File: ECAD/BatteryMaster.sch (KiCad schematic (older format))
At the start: 33 parts

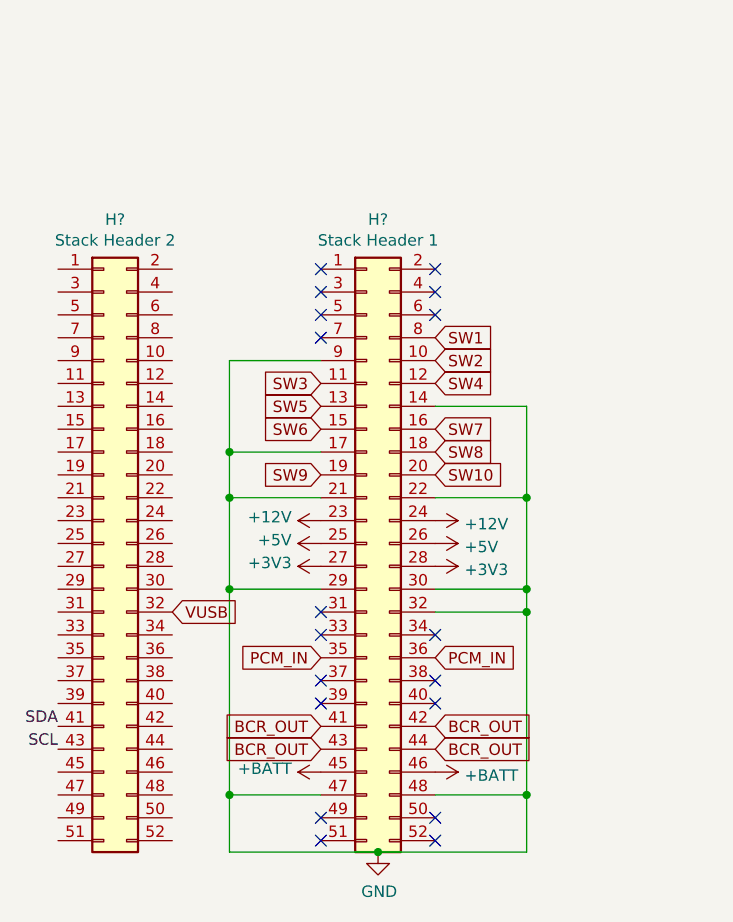
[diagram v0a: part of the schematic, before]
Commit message: rearrange the stack headers to make some damn sense *looks at clydespace*
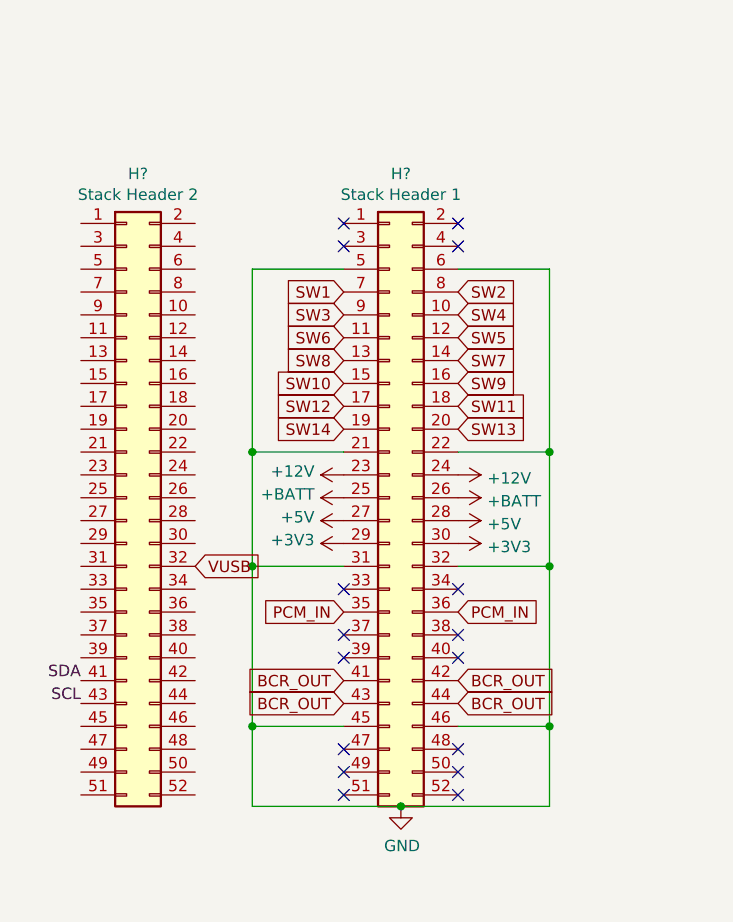
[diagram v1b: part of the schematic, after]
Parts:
- removed H?: Stack Header 2, symbol Connector_Generic:Conn_02x26_Odd_Even
- removed H?: Stack Header 1, symbol Connector_Generic:Conn_02x26_Odd_Even
- added H?: Stack Header 2, symbol Connector_Generic:Conn_02x26_Odd_Even
- added H?: Stack Header 1, symbol Connector_Generic:Conn_02x26_Odd_Even
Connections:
- net +12V: now also H?.23 (Pin_23), H?.24 (Pin_24)
- net +3V3: now also H?.29 (Pin_29), H?.30 (Pin_30)
- net +5V: now also H?.27 (Pin_27), H?.28 (Pin_28)
- net +BATT: now also H?.25 (Pin_25), H?.26 (Pin_26)
- net BCR_OUT: now also H?.41 (Pin_41), H?.42 (Pin_42), H?.43 (Pin_43), H?.44 (Pin_44)
- net GND: now also H?.21 (Pin_21), H?.22 (Pin_22), H?.31 (Pin_31), H?.32 (Pin_32), H?.45 (Pin_45), H?.46 (Pin_46), H?.5 (Pin_5), H?.6 (Pin_6)
- net PCM_IN: now also H?.35 (Pin_35), H?.36 (Pin_36)
- net SCL: now also H?.43 (Pin_43)
- net SDA: now also H?.41 (Pin_41)
- net SW1: now also H?.7 (Pin_7)
- net SW10: now also H?.15 (Pin_15)
- net SW2: now also H?.8 (Pin_8)
- net SW3: now also H?.9 (Pin_9)
- net SW4: now also H?.10 (Pin_10)
- net SW5: now also H?.12 (Pin_12)
- net SW6: now also H?.11 (Pin_11)
- net SW7: now also H?.14 (Pin_14)
- net SW8: now also H?.13 (Pin_13)
- net SW9: now also H?.16 (Pin_16)
- net VUSB: now also H?.32 (Pin_32)
- new net SW11: H?.18 (Pin_18)
- new net SW12: H?.17 (Pin_17)
- new net SW13: H?.20 (Pin_20)
- new net SW14: H?.19 (Pin_19)
- no-connect marks 18 -> 16

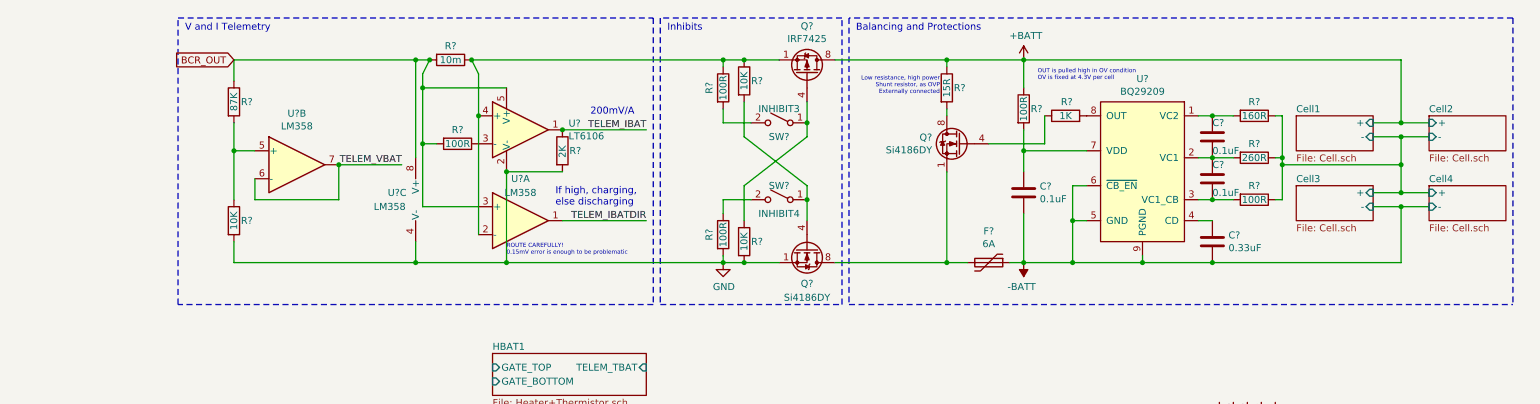
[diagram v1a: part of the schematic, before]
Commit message: spec out new cell protection IC and mosfets, figured out current limit calculation
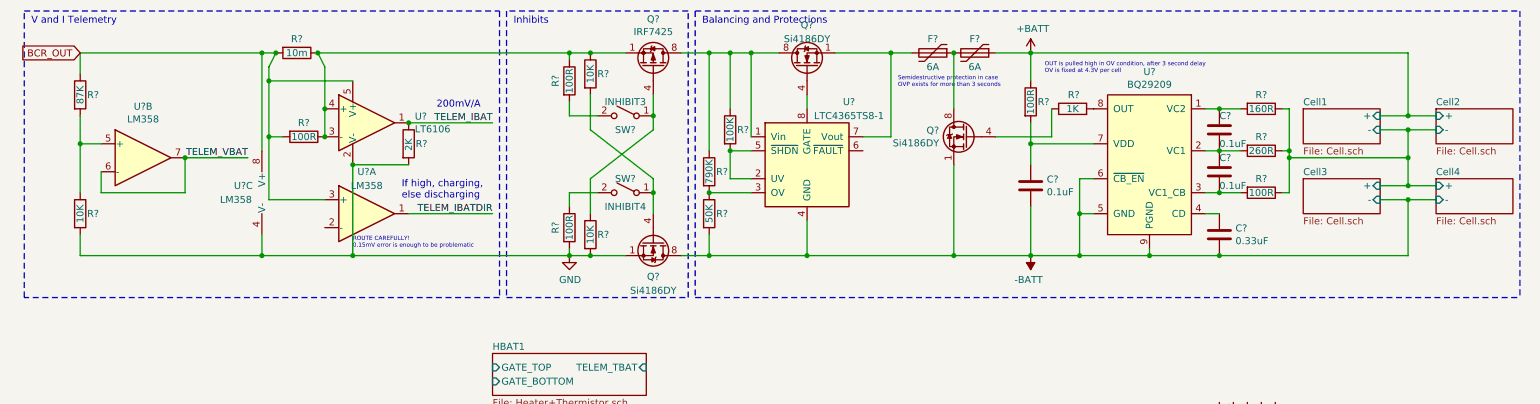
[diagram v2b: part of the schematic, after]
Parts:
- removed R?: 15R, symbol Device:R
- added F?: 6A, symbol Device:Polyfuse
- added Q?: Si4186DY, Package_SO:SOIC-8_3.9x4.9mm_P1.27mm, symbol Transistor_FET:Si4162DY
- added R?: 100K, symbol Device:R
- added R?: 790K, symbol Device:R
- added R?: 50K, symbol Device:R
- added U?: LTC4365TS8-1, symbol Power_Management:LTC4365TS8-1
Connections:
- net +BATT: now also F?.1; no longer Q?.5 (D), Q?.6 (D), Q?.7 (D), Q?.8 (D)
- net -BATT: now also Q?.1 (S), Q?.2 (S), Q?.3 (S), Q?.5 (D), Q?.6 (D), Q?.7 (D), Q?.8 (D), R?.2, U?.4 (GND); no longer F?.1
- net at Q?.5 (D), Q?.6 (D), Q?.7 (D)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: now also F?.2, F?.1
- net at Q?.1 (S), Q?.2 (S), Q?.3 (S)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: now also R?.1, U?.3 (-); no longer U?.2 (-)
- new net: F?.2, Q?.1 (S), Q?.2 (S), Q?.3 (S), U?.7 (Vout)
- new net: Q?.5 (D), Q?.5 (D), Q?.6 (D), Q?.6 (D), Q?.7 (D), Q?.7 (D), Q?.8 (D), Q?.8 (D), R?.1, R?.1, U?.1 (Vin)
- new net: R?.2, U?.2 (UV), U?.5 (~SHDN)
- new net: R?.1, R?.2, U?.3 (OV)
- new net: Q?.4 (G), U?.8 (GATE)
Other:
- note added: "OUT is pulled high in OV condition, after 3 second delay\nOV is fixed at 4.3V per cell"
- note added: "Semidestructive protection in case \nOVP exists for more than 3 seconds"
- note removed: "Low resistance, high power\nShunt resistor, as OVP\nExternally connected"
- note removed: "OUT is pulled high in OV condition\nOV is fixed at 4.3V per cell"
- moved on the sheet: C?, F?, Q?, R?, SW?, U?, U?A, U?B, U?C

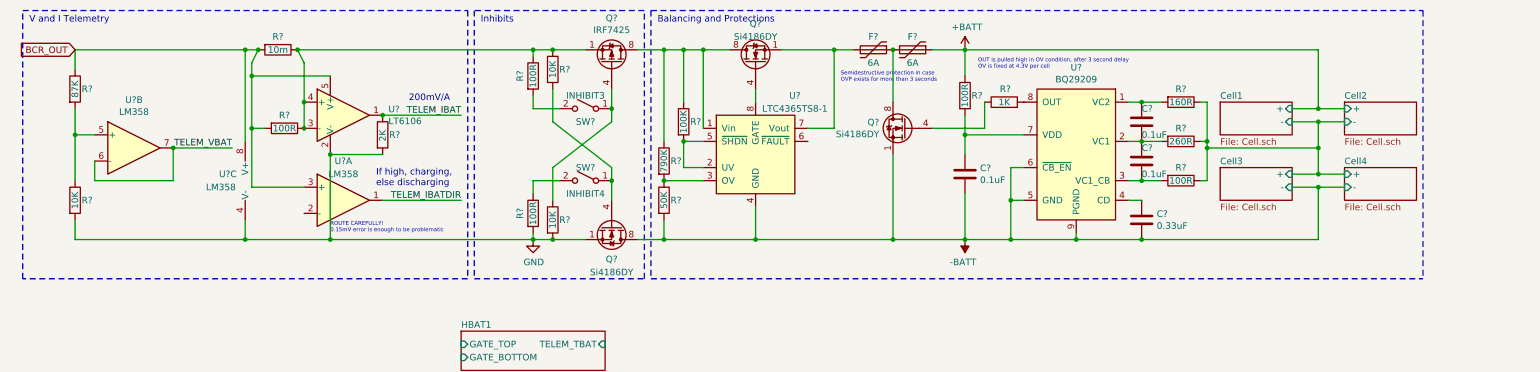
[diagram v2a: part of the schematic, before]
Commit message: Add OCP, resize some sheets
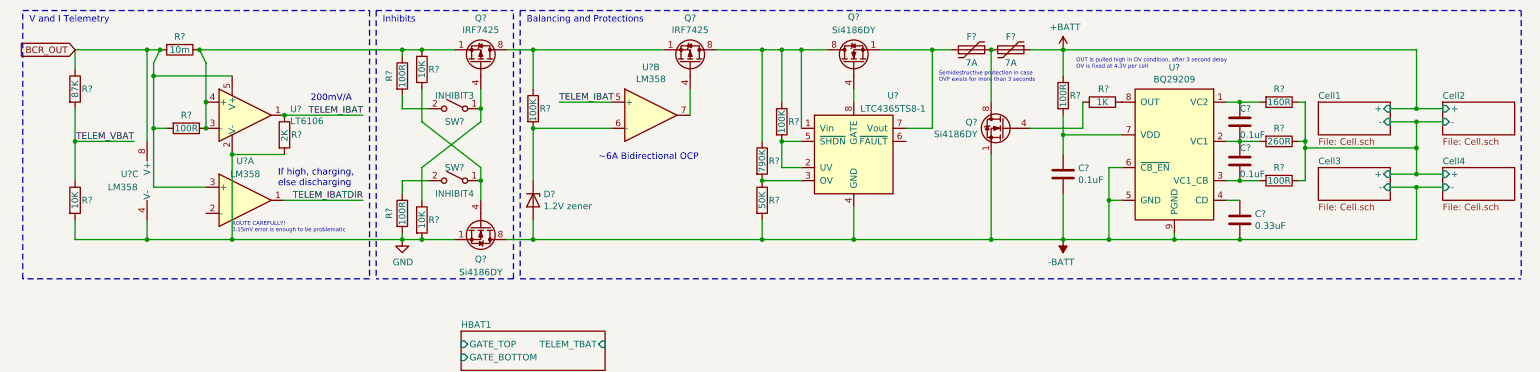
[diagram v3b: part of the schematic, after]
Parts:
- added D?: 1.2V zener, symbol Device:D_Zener
- added Q?: IRF7425, Package_SO:SOIC-8_3.9x4.9mm_P1.27mm, symbol Transistor_FET:IRF7404
- added R?: 100K, symbol Device:R
- F? (x2): value 6A -> 7A
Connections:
- net -BATT: now also D?.2 (A)
- net TELEM_IBAT: now also U?.5 (+)
- net TELEM_VBAT: now also R?.1, R?.2; no longer U?.6 (-), U?.7
- net at Q?.5 (D), Q?.6 (D), Q?.7 (D)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: now also Q?.5 (D), Q?.6 (D), Q?.7 (D), Q?.8 (D); no longer Q?.5 (D), Q?.6 (D), Q?.7 (D), Q?.8 (D)
- new net: Q?.1 (S), Q?.2 (S), Q?.3 (S), Q?.5 (D), Q?.6 (D), Q?.7 (D), Q?.8 (D), R?.1
- new net: D?.1 (K), R?.2, U?.6 (-)
- new net: Q?.4 (G), U?.7
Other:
- note added: "~~6A Bidirectional OCP"
- moved on the sheet: C?, F?, Q?, R?, SW?, U?, U?A, U?B, U?C

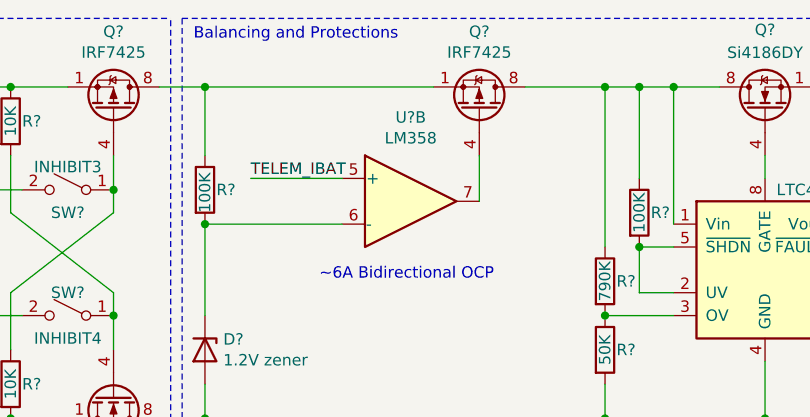
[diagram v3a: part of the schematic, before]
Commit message: fix the bidirectional ocp to actually be bidirectional
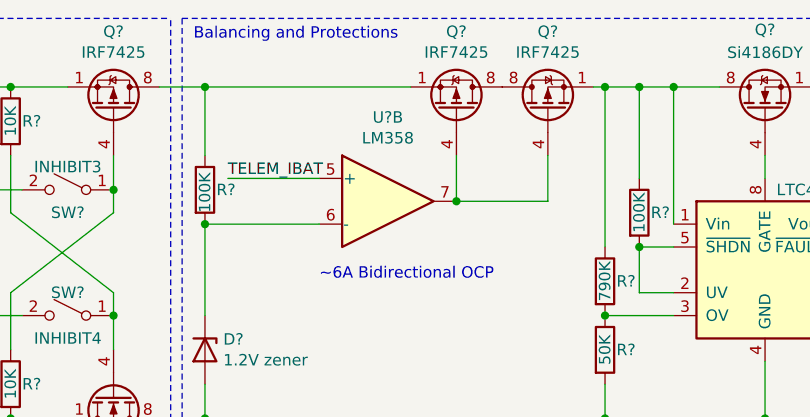
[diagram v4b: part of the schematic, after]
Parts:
- added Q?: IRF7425, Package_SO:SOIC-8_3.9x4.9mm_P1.27mm, symbol Transistor_FET:IRF7404
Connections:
- net at Q?.5 (D), Q?.6 (D), Q?.7 (D)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: now also Q?.1 (S), Q?.2 (S), Q?.3 (S); no longer Q?.5 (D), Q?.6 (D), Q?.7 (D), Q?.8 (D)
- net at Q?.4 (G), U?.7: now also Q?.4 (G)
- new net: Q?.5 (D), Q?.5 (D), Q?.6 (D), Q?.6 (D), Q?.7 (D), Q?.7 (D), Q?.8 (D), Q?.8 (D)
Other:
- moved on the sheet: Q?, U?B
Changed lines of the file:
@@
 L Amplifier_Operational:LM358 U?
 U 2 1 61DFA6F3
-P 5300 1300
-F 0 "U?" H 5300 1667 50  0000 C CNN
-F 1 "LM358" H 5300 1576 50  0000 C CNN
-F 2 "" H 5300 1300 50  0001 C CNN
-F 3 "http://www.ti.com/lit/ds/symlink/lm2904-n.pdf" H 5300 1300 50  0001 C CNN
-	2    5300 1300
+P 5200 1300
+F 0 "U?" H 5200 1667 50  0000 C CNN
+F 1 "LM358" H 5200 1576 50  0000 C CNN
+F 2 "" H 5200 1300 50  0001 C CNN
+F 3 "http://www.ti.com/lit/ds/symlink/lm2904-n.pdf" H 5200 1300 50  0001 C CNN
+	2    5200 1300
 	1    0    0    -1
 $EndComp
@@
 	4400 1100 4400 800
 Connection ~ 4400 1400
-Text Label 4600 1200 0    50   ~ 0
+Text Label 4500 1200 0    50   ~ 0
 TELEM_IBAT
 Wire Wire Line
-	4600 1200 5000 1200
-Wire Wire Line
-	4400 800  5400 800
+	4500 1200 4900 1200
+Wire Wire Line
+	4400 800  5300 800
 Wire Wire Line
 	6850 1100 6850 1200
@@
 L Transistor_FET:IRF7404 Q?
 U 1 1 622A211E
-P 5600 900
-F 0 "Q?" V 5942 900 50  0000 C CNN
-F 1 "IRF7425" V 5851 900 50  0000 C CNN
-F 2 "Package_SO:SOIC-8_3.9x4.9mm_P1.27mm" H 5800 825 50  0001 L CIN
-F 3 "http://www.infineon.com/dgdl/irf7404.pdf?fileId=5546d462533600a4015355fa2b5b1b9e" V 5600 900 50  0001 L CNN
-	1    5600 900
+P 5500 900
+F 0 "Q?" V 5842 900 50  0000 C CNN
+F 1 "IRF7425" V 5751 900 50  0000 C CNN
+F 2 "Package_SO:SOIC-8_3.9x4.9mm_P1.27mm" H 5700 825 50  0001 L CIN
+F 3 "http://www.infineon.com/dgdl/irf7404.pdf?fileId=5546d462533600a4015355fa2b5b1b9e" V 5500 900 50  0001 L CNN
+	1    5500 900
 	0    1    -1   0
 $EndComp
-Wire Wire Line
-	4400 1400 5000 1400
 Connection ~ 4400 800
 Wire Wire Line
-	5600 1300 5600 1100
-Wire Wire Line
-	5800 800  6150 800
-Connection ~ 6150 800
+	5500 1300 5500 1100
 Wire Wire Line
 	4400 2250 6150 2250
@@
 Wire Notes Line
 	500  500  3150 500
+$Comp
+L Transistor_FET:IRF7404 Q?
+U 1 1 61CCE42A
+P 5900 900
+F 0 "Q?" V 6242 900 50  0000 C CNN
+F 1 "IRF7425" V 6151 900 50  0000 C CNN
+F 2 "Package_SO:SOIC-8_3.9x4.9mm_P1.27mm" H 6100 825 50  0001 L CIN
+F 3 "http://www.infineon.com/dgdl/irf7404.pdf?fileId=5546d462533600a4015355fa2b5b1b9e" V 5900 900 50  0001 L CNN
+	1    5900 900
+	0    -1   -1   0
+$EndComp
+Wire Wire Line
+	4400 1400 4900 1400
+Wire Wire Line
+	5900 1100 5900 1300
+Wire Wire Line
+	5900 1300 5500 1300
+Connection ~ 5500 1300
+Wire Wire Line
+	6150 800  6100 800
+Connection ~ 6150 800
 $EndSCHEMATC
